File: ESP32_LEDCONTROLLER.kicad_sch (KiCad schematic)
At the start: 20 parts, among them J1 ST-04, J2 ST-00, J3 ST-01, J4 ST-02, J5 ST-03, U1 LM2576HVT-5, U2 ESP32_NODEMCU, U3 SN74LV4T125

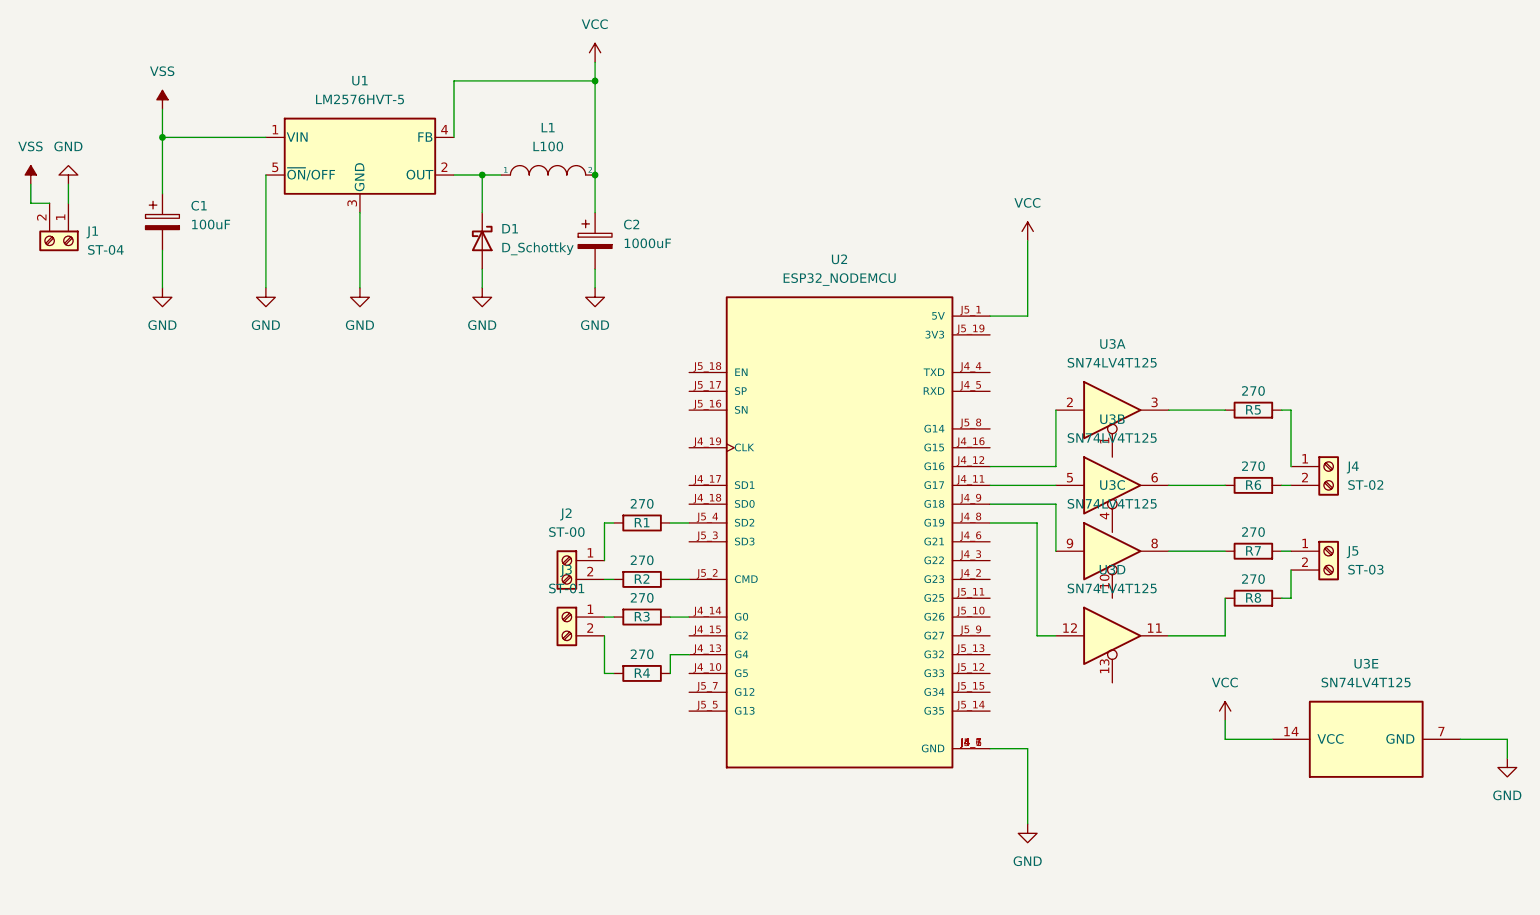
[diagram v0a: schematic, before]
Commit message: v0.1 of the LED Controller has been completed.
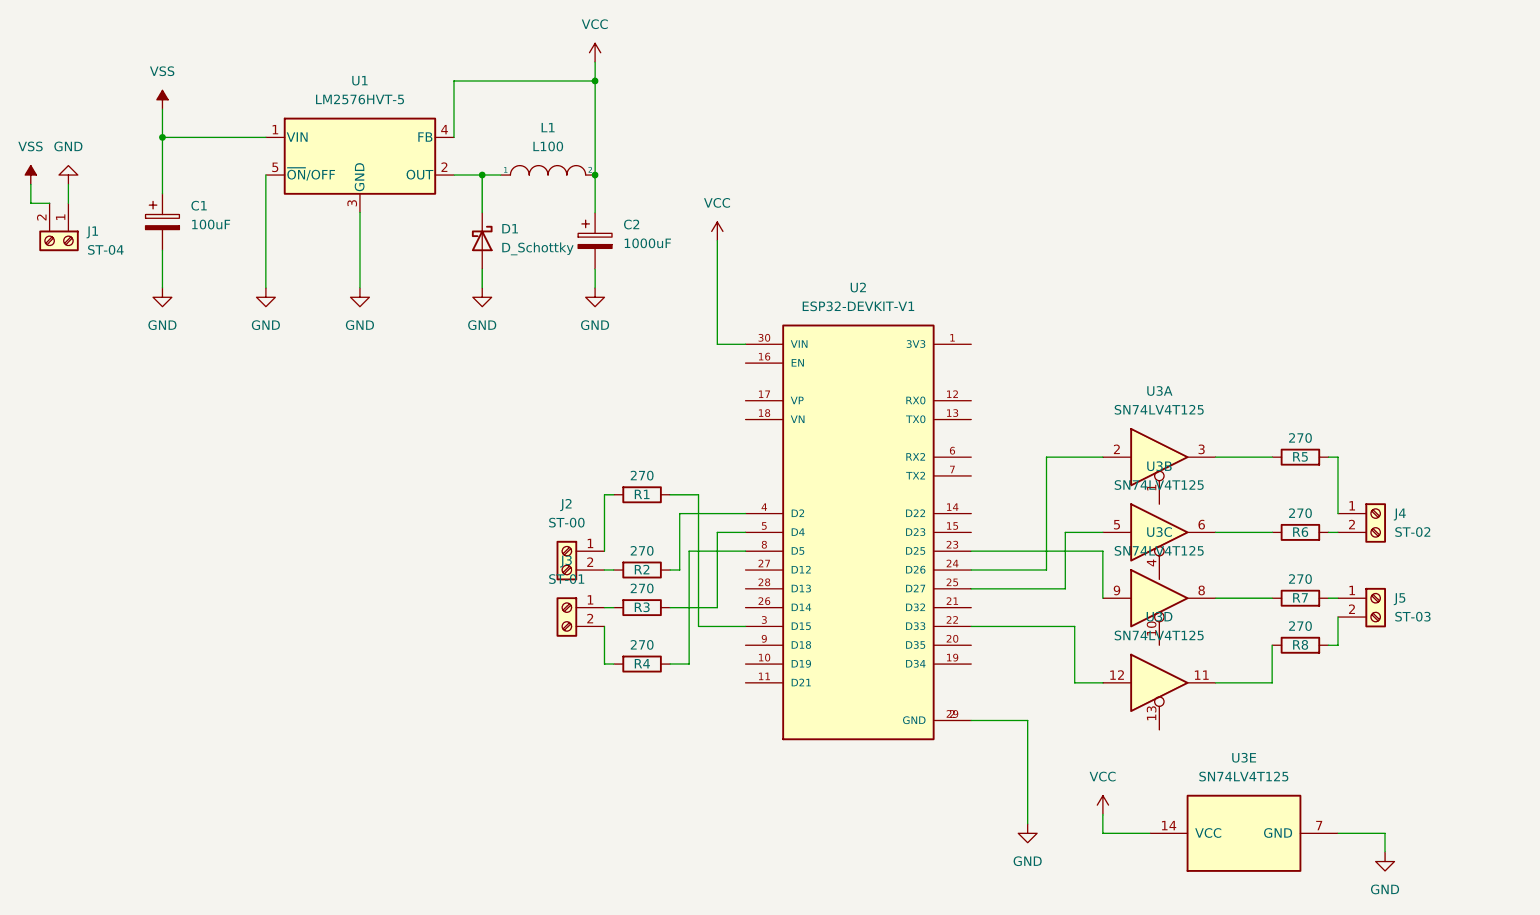
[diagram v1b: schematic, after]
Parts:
- removed U2: ESP32_NODEMCU, Esp32NodeMCU:MODULE_ESP32_NODEMCU, symbol ESP32_NODEMCU:ESP32_NODEMCU
- added U2: ESP32-DEVKIT-V1, MODULE_ESP32_DEVKIT_V1, symbol ESP32-DEVKIT-V1:ESP32-DEVKIT-V1
- U3: footprint (none) -> Package_DIP:DIP-14_W7.62mm
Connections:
- net GND: now also U2.2 (GND), U2.29 (GND)
- net VCC: now also U2.30 (VIN)
- net at U3.2: now also U2.24 (D26)
- net at U3.5: now also U2.25 (D27)
- net at R4.1: now also U2.8 (D5)
- net at R3.1: now also U2.5 (D4)
- net at U3.12: now also U2.22 (D33)
- net at U3.9: now also U2.23 (D25)
- net at R2.1: now also U2.4 (D2)
- net at R1.1: now also U2.3 (D15)
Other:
- moved on the sheet: J2, J3, J4, J5, R1, R2, R3, R4, R5, R6, R7, R8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
